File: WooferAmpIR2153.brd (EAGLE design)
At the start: 142.2 x 47.3 mm, 70 parts

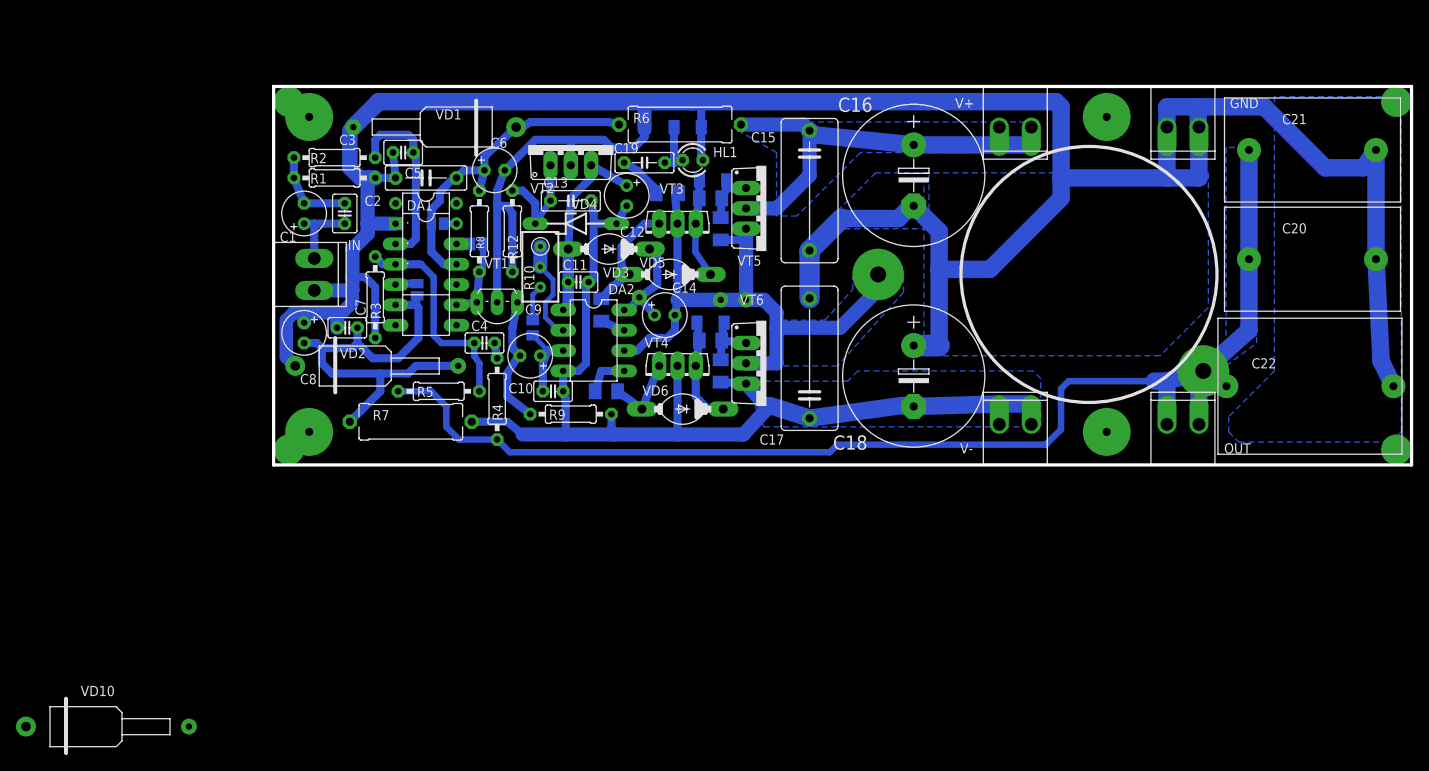
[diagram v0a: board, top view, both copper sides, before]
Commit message: h1
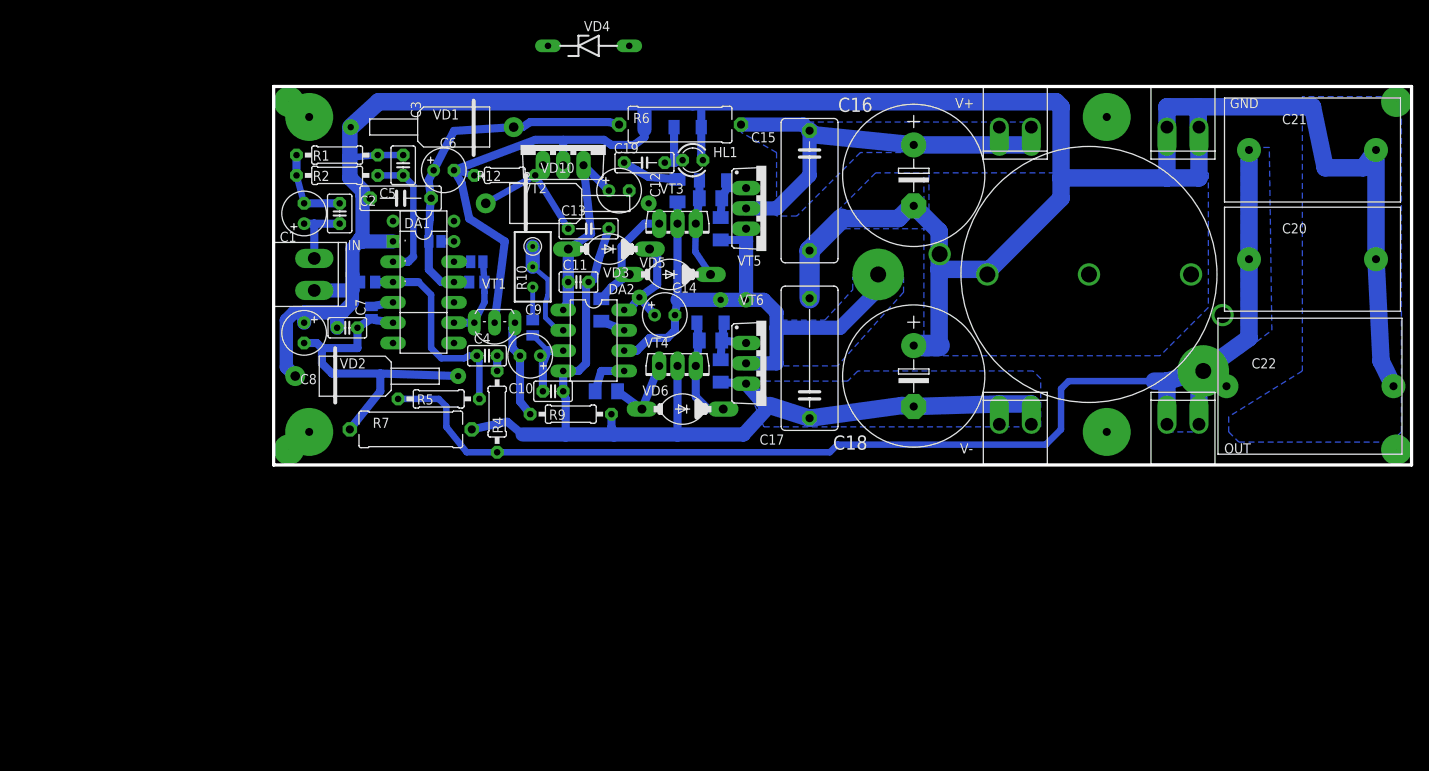
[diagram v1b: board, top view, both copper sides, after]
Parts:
- added U$1: L-D30, woofer:L-D30
- R12: device resistor:0207/10 -> resistor:0204/7
- R3, R8: device resistor:0207/10 -> resistor:M0805
- moved VD10 87.1 mm to (34.0, 31.1)
- moved VD4 22.3 mm to (38.7, 50.8)
- moved R12 7.05 mm to (28.3, 34.6), turned to 0 degrees
- moved SJ1 6.39 mm to (11.6, 17.5)
- moved R8 6.36 mm to (24.8, 21.3), flipped to the bottom, turned to 0 degrees
- moved C6 6.35 mm to (20.6, 35.2)
- moved C13 4.14 mm to (38.7, 27.9)
- moved C5 4.07 mm to (15.2, 31.8)
- moved R1 2.88 mm to (7.30, 37.1)
- moved VT1 2.56 mm to (27.0, 16.2)
- moved DA1 2.25 mm to (18.1, 21.3)
- moved SJ3 2.25 mm to (19.5, 26.4)
- moved R2 2.25 mm to (7.30, 34.6)
- moved SJ2 2.22 mm to (24.8, 23.8)
- moved R3 2.13 mm to (11.1, 21.3), flipped to the bottom, turned to 180 degrees
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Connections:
- net N$21 renamed L-OUT
- net GND: now also U$1.1A, U$1.1B, U$1.2B, U$1.D
- net N$2: now also VD10.C; no longer VD4.C
- net V-: now also VD10.A; no longer VD4.A
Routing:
- net VC-: track 54.0 -> 42.1 mm
- net V-: track 133.8 -> 125.3 mm
- net C+: track 22.8 -> 16.7 mm
- net N$50: track 17.2 -> 13.0 mm
- net VC+: track 41.2 -> 44.7 mm
- net N$2: track 13.9 -> 16.5 mm
- net N$9: track 5.64 -> 7.16 mm
- net NL: track 76.8 -> 75.4 mm
- net C-: track 27.4 -> 26.1 mm
- net N$37: track 2.83 -> 4.04 mm
- net N$19: track 9.43 -> 8.79 mm
